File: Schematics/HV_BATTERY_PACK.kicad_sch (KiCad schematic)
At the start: 6 parts

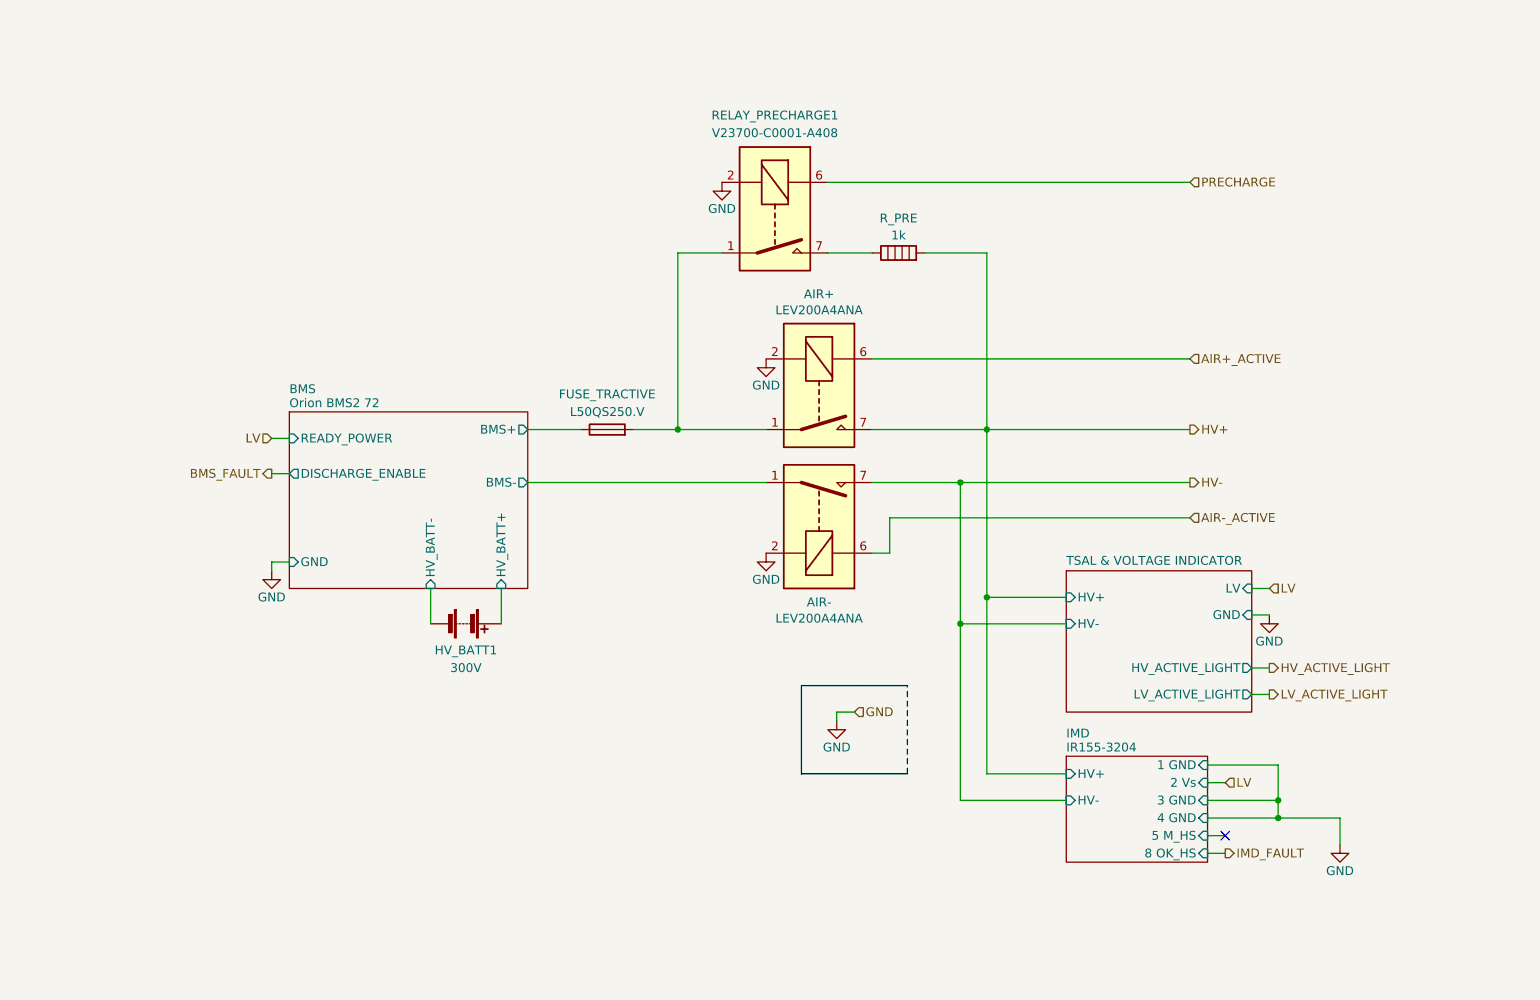
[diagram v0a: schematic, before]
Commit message: REFACTOR
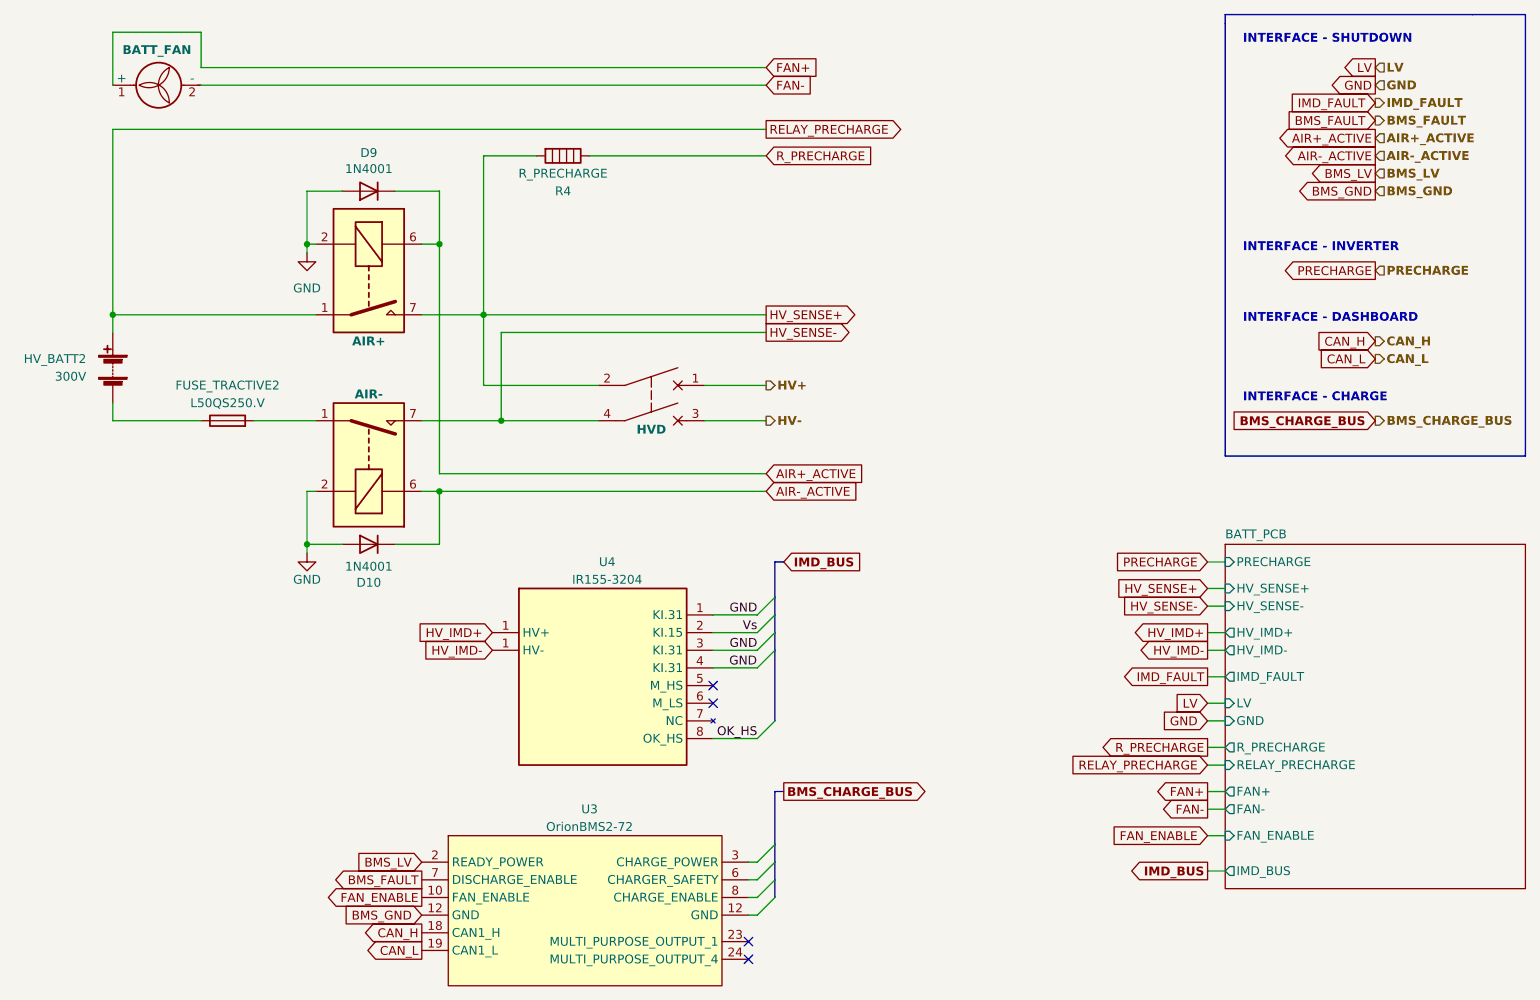
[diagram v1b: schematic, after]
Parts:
- removed FUSE_TRACTIVE: L50QS250.V, symbol Device:Fuse
- removed HV_BATT1: 300V, symbol Device:Battery
- removed RELAY_PRECHARGE1: V23700-C0001-A408, Relay_THT:Relay_StandexMeder_DIP_LowProfile, symbol Relay:DIPxx-1Axx-12x
- removed R_PRE: 1k, symbol Device:Heater
- added CB2: HVD, symbol Device:CircuitBreaker_2P
- added D10, D9: 1N4001, Diode_THT:D_DO-41_SOD81_P10.16mm_Horizontal, symbol Diode:1N4001
- added FUSE_TRACTIVE2: L50QS250.V, symbol Device:Fuse
- added HV_BATT2: 300V, symbol Device:Battery
- added M4: BATT_FAN, symbol Motor:Fan
- added R4: R_PRECHARGE, symbol Device:Heater
- added U3: OrionBMS2-72, symbol A-FA_PARTS:OrionBMS2-72
- added U4: IR155-3204, symbol A-FA_PARTS:IR155-3204
- AIR+2: renamed from AIR+; value LEV200A4ANA -> AIR+
- AIR-2: renamed from AIR-; value LEV200A4ANA -> AIR-
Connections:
- net AIR+_ACTIVE: now also D9.1 (K)
- net AIR-_ACTIVE: now also D10.1 (K)
- net BMS_FAULT: now also U3.7 (DISCHARGE_ENABLE)
- net GND: now also D10.2 (A), D9.2 (A), U4.1 (KI.31), U4.3 (KI.31), U4.4 (KI.31)
- net HV+: now also CB2.1; no longer AIR+2.7, AIR+2.8
- net HV-: now also CB2.3; no longer AIR-2.7, AIR-2.8
- net RELAY_PRECHARGE: now reaches AIR+2.1, AIR+2.14
- net RELAY_PRECHARGE: now also HV_BATT2.1 (+)
- net BMS/BMS-: no longer names the net of AIR-2.1, AIR-2.14
- net BMS/BMS-: now also FUSE_TRACTIVE2.2
- new net: FUSE_TRACTIVE2.1, HV_BATT2.2 (-)
- new net BMS_GND: U3.12 (GND)
- new net BMS_LV: U3.2 (READY_POWER)
- new net CAN_H: U3.18 (CAN1_H)
- new net CAN_L: U3.19 (CAN1_L)
- new net FAN+: M4.1 (+)
- new net FAN-: M4.2 (-)
- new net FAN_ENABLE: U3.10 (FAN_ENABLE)
- new net HV_IMD+: U4.1 (KI.31)
- new net HV_IMD-: U4.1 (KI.31)
- new net HV_SENSE+: AIR+2.7, AIR+2.8, CB2.2, R4.2
- new net HV_SENSE-: AIR-2.7, AIR-2.8, CB2.4
- new net OK_HS: U4.8 (OK_HS)
- new net R_PRECHARGE: R4.1
- new net Vs: U4.2 (KI.15)
- no-connect marks 1 -> 4
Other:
- removed sheet BMS
- removed sheet IMD
- removed sheet TSAL & VOLTAGE INDICATOR
- added sheet BATT_PCB (BATT_PCB.kicad_sch)
- note added: "INTERFACE - CHARGE"
- note added: "INTERFACE - DASHBOARD"
- note added: "INTERFACE - INVERTER"
- note added: "INTERFACE - SHUTDOWN"
